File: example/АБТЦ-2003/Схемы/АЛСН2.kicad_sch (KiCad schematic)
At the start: 21 parts

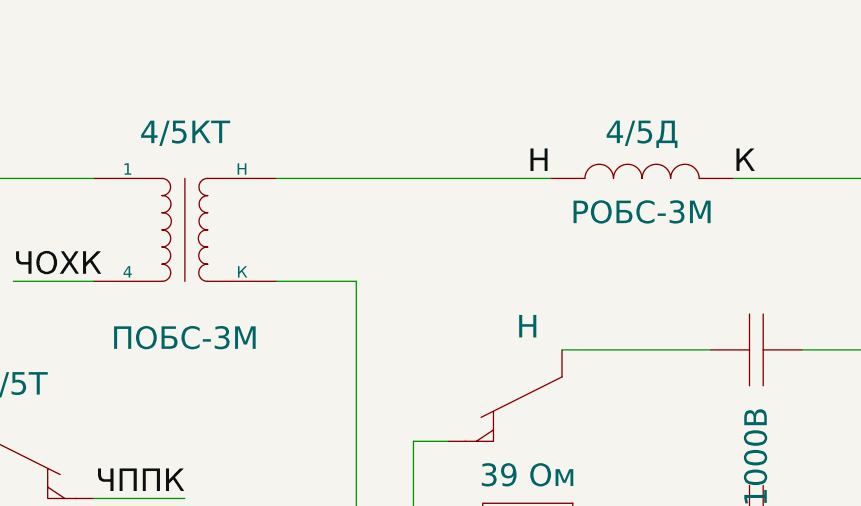
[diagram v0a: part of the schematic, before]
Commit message: Обновление примера
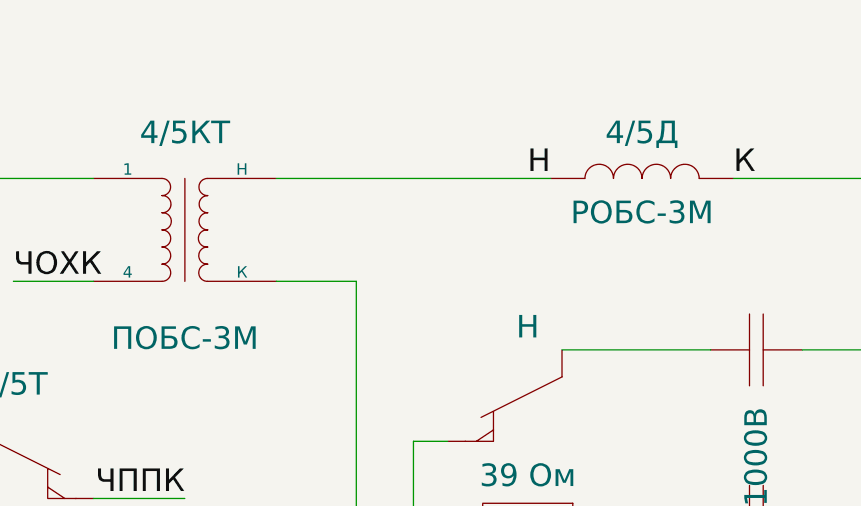
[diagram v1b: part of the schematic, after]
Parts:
- Н11, Н111, Н1111, Н111111, Н11112, Н111212, Н11122, Н1114, Н1115, Н1116, Н113: symbol SCB_Relay:Контакт_нейтрального_якоря -> SCB_Legacy:Контакт_нейтрального_якоря_бн
- Н1111111: symbol SCB_Relay:Контакт_нейтрального_якоря_НЗ -> SCB_Legacy:Контакт_нейтрального_якоря_НЗ_бн
